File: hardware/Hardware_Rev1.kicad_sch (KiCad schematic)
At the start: 146 parts, among them J1 RJ45_LED_Shielded, J2 6P6C, Q1 BSS138, Q10 AO3401A, Q11 AO3401A, Q12 AO3401A, Q13 BSS138, Q14 BSS138, Q15 BSS138, Q16 AO3401A, Q17 AO3401A, Q18 AO3401A, Q19 BSS138, Q2 BSS138, Q20 BSS138, Q21 BSS138, Q22 AO3401A, Q23 AO3401A, Q24 AO3401A, Q3 BSS138, Q4 AO3401A, Q5 AO3401A, Q6 AO3401A, Q7 BSS138, Q8 BSS138, Q9 BSS138, U1 OKI, U2 Teensy4.1_DEV-16771

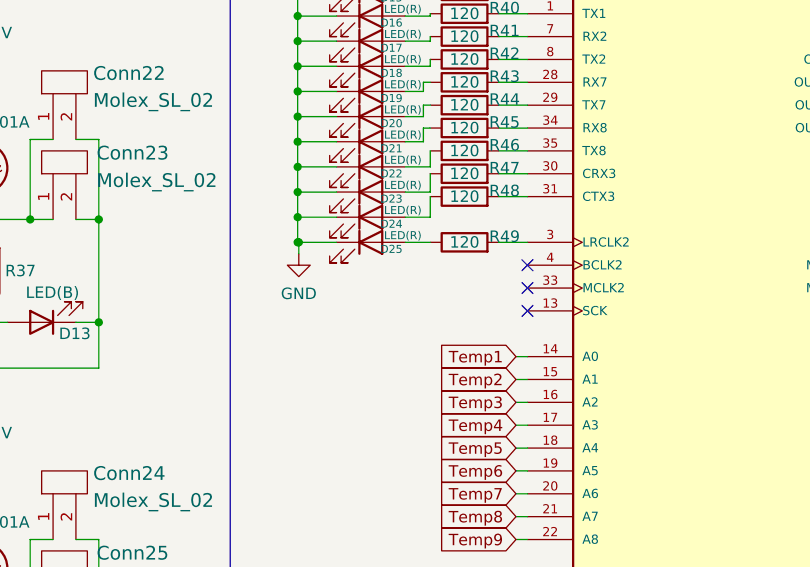
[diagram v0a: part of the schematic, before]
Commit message: Finished connections
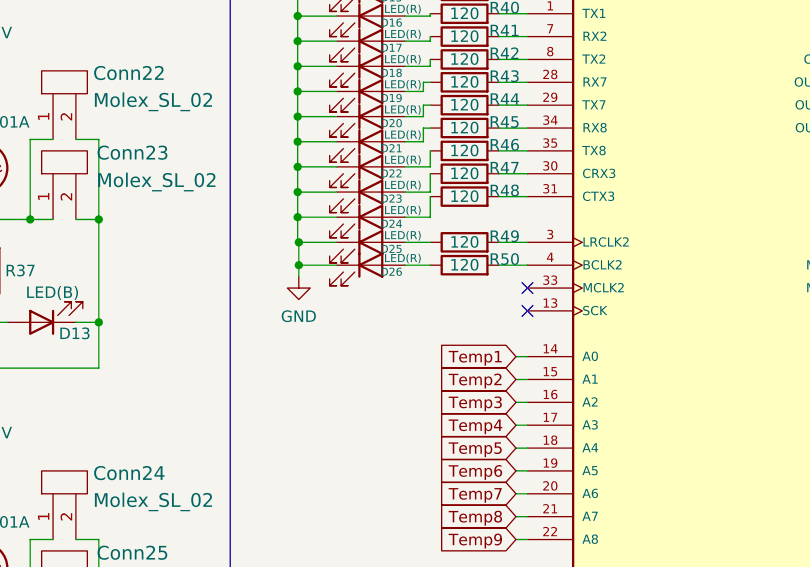
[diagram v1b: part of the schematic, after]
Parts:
- added D26: LED(R), LED_SMD:LED_0603_1608Metric_Pad1.05x0.95mm_HandSolder, symbol Device:LED
- added R50: 120, Resistor_SMD:R_0603_1608Metric_Pad0.98x0.95mm_HandSolder, symbol Device:R
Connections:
- net GND: now also D26.1 (K)
- net at U2.4 (BCLK2): now also R50.2
- new net: D26.2 (A), R50.1
- no-connect marks 23 -> 22
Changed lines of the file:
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@@
   (junction (at 187.833 77.216) (diameter 0) (color 0 0 0 0)
   )
+  (junction (at 187.96 82.55) (diameter 0) (color 0 0 0 0)
+  )
   (junction (at 73.66 63.5) (diameter 0) (color 0 0 0 0)
   )
@@
   (junction (at 102.235 93.98) (diameter 0) (color 0 0 0 0)
   )
-  (junction (at 187.96 80.01) (diameter 0) (color 0 0 0 0)
-  )
   (junction (at 125.095 167.005) (diameter 0) (color 0 0 0 0)
   )
@@
   (junction (at 33.655 63.5) (diameter 0) (color 0 0 0 0)
   )
-  (junction (at 187.833 80.01) (diameter 0) (color 0 0 0 0)
-  )
   (junction (at 153.035 153.035) (diameter 0) (color 0 0 0 0)
   )
@@
   (junction (at 45.72 121.92) (diameter 0) (color 0 0 0 0)
   )
+  (junction (at 187.96 80.01) (diameter 0) (color 0 0 0 0)
+  )
   (junction (at 22.225 116.205) (diameter 0) (color 0 0 0 0)
   )
@@
   (no_connect (at 254 31.75))
   (no_connect (at 254 29.21))
-  (no_connect (at 213.36 82.55))
   (no_connect (at 254 77.47))
   (no_connect (at 254 74.93))
@@
     (stroke (width 0) (type default) (color 0 0 0 0))
   )
+  (wire (pts (xy 187.96 80.01) (xy 187.96 82.55))
+    (stroke (width 0) (type default) (color 0 0 0 0))
+  )
   (wire (pts (xy 118.11 68.58) (xy 120.65 68.58))
     (stroke (width 0) (type default) (color 0 0 0 0))
@@
     (stroke (width 0) (type default) (color 0 0 0 0))
   )
+  (wire (pts (xy 192.151 82.55) (xy 187.96 82.55))
+    (stroke (width 0) (type default) (color 0 0 0 0))
+  )
   (wire (pts (xy 153.67 60.325) (xy 153.67 63.5))
     (stroke (width 0) (type default) (color 0 0 0 0))
@@
     (stroke (width 0) (type default) (color 0 0 0 0))
   )
+  (wire (pts (xy 199.771 82.55) (xy 202.565 82.55))
+    (stroke (width 0) (type default) (color 0 0 0 0))
+  )
   (wire (pts (xy 85.725 77.47) (xy 85.725 68.58))
     (stroke (width 0) (type default) (color 0 0 0 0))
@@
     (stroke (width 0) (type default) (color 0 0 0 0))
   )
-  (wire (pts (xy 187.96 80.01) (xy 187.833 80.01))
-    (stroke (width 0) (type default) (color 0 0 0 0))
-  )
   (wire (pts (xy 153.035 178.435) (xy 154.94 178.435))
     (stroke (width 0) (type default) (color 0 0 0 0))
@@
     (stroke (width 0) (type default) (color 0 0 0 0))
   )
+  (wire (pts (xy 210.185 82.55) (xy 213.36 82.55))
+    (stroke (width 0) (type default) (color 0 0 0 0))
+  )
   (wire (pts (xy 42.545 167.005) (xy 45.085 167.005))
     (stroke (width 0) (type default) (color 0 0 0 0))
@@
     (stroke (width 0) (type default) (color 0 0 0 0))
   )
-  (wire (pts (xy 187.96 80.01) (xy 187.96 81.28))
+  (wire (pts (xy 187.96 82.55) (xy 187.96 83.82))
     (stroke (width 0) (type default) (color 0 0 0 0))
   )
@@
     (stroke (width 0) (type default) (color 0 0 0 0))
   )
-  (wire (pts (xy 192.151 80.01) (xy 187.96 80.01))
+  (wire (pts (xy 187.833 80.01) (xy 187.96 80.01))
     (stroke (width 0) (type default) (color 0 0 0 0))
   )
@@
     (stroke (width 0) (type default) (color 0 0 0 0))
   )
+  (wire (pts (xy 187.96 80.01) (xy 192.151 80.01))
+    (stroke (width 0) (type default) (color 0 0 0 0))
+  )
   (wire (pts (xy 33.655 131.445) (xy 33.655 133.35))
     (stroke (width 0) (type default) (color 0 0 0 0))
@@
     (pin "1")
   )
+  (symbol (lib_id "Device:LED") (at 195.961 82.55 0) (unit 1)
+    (in_bom yes) (on_board yes)
+    (property "Reference" "D26" (id 0) (at 198.247 83.312 0)
+      (effects (font (size 0.889 0.889)))
+    )
+    (property "Value" "LED(R)" (id 1) (at 199.517 81.788 0)
+      (effects (font (size 0.889 0.889)))
+    )
+    (property "Footprint" "LED_SMD:LED_0603_1608Metric_Pad1.05x0.95mm_HandSolder" (id 2) (at 195.961 82.55 0)
+      (effects (font (size 1.27 1.27)) hide)
+    )
+    (property "Datasheet" "~" (id 3) (at 195.961 82.55 0)
+      (effects (font (size 1.27 1.27)) hide)
+    )
+    (pin "1")
+    (pin "2")
+  )
   (symbol (lib_id "power:GND") (at 337.82 89.535 0) (unit 1)
     (in_bom yes) (on_board yes) (fields_autoplaced)
@@
     (pin "1")
   )
-  (symbol (lib_id "power:GND") (at 187.96 81.28 0) (unit 1)
+  (symbol (lib_id "power:GND") (at 187.96 83.82 0) (unit 1)
     (in_bom yes) (on_board yes) (fields_autoplaced)
-    (property "Reference" "#PWR031" (id 0) (at 187.96 87.63 0)
+    (property "Reference" "#PWR031" (id 0) (at 187.96 90.17 0)
       (effects (font (size 1.27 1.27)) hide)
     )
-    (property "Value" "GND" (id 1) (at 187.96 85.7234 0))
-    (property "Footprint" "" (id 2) (at 187.96 81.28 0)
+    (property "Value" "GND" (id 1) (at 187.96 88.2634 0))
+    (property "Footprint" "" (id 2) (at 187.96 83.82 0)
       (effects (font (size 1.27 1.27)) hide)
     )
-    (property "Datasheet" "" (id 3) (at 187.96 81.28 0)
+    (property "Datasheet" "" (id 3) (at 187.96 83.82 0)
       (effects (font (size 1.27 1.27)) hide)
     )
@@
     (pin "2")
   )
+  (symbol (lib_id "Device:R") (at 206.375 82.55 90) (unit 1)
+    (in_bom yes) (on_board yes)
+    (property "Reference" "R50" (id 0) (at 210.82 81.915 90))
+    (property "Value" "120" (id 1) (at 206.375 82.55 90))
+    (property "Footprint" "Resistor_SMD:R_0603_1608Metric_Pad0.98x0.95mm_HandSolder" (id 2) (at 206.375 84.328 90)
+      (effects (font (size 1.27 1.27)) hide)
+    )
+    (property "Datasheet" "~" (id 3) (at 206.375 82.55 0)
+      (effects (font (size 1.27 1.27)) hide)
+    )
+    (pin "1")
+    (pin "2")
+  )
   (symbol (lib_id "Device:LED") (at 39.37 88.9 180) (unit 1)
     (in_bom yes) (on_board yes)
@@
       (reference "D25") (unit 1) (value "LED(R)") (footprint "LED_SMD:LED_0603_1608Metric_Pad1.05x0.95mm_HandSolder")
     )
+    (path "/6d949603-847f-4e56-b193-01912840b2f5"
+      (reference "D26") (unit 1) (value "LED(R)") (footprint "LED_SMD:LED_0603_1608Metric_Pad1.05x0.95mm_HandSolder")
+    )
     (path "/c2380cb7-4961-4052-bc8b-0b990bf9ca9f"
       (reference "J1") (unit 1) (value "RJ45_LED_Shielded") (footprint "MRDT_Connectors:RJ45_Teensy")
@@
       (reference "R49") (unit 1) (value "120") (footprint "Resistor_SMD:R_0603_1608Metric_Pad0.98x0.95mm_HandSolder")
     )
+    (path "/a6972e9c-2b36-4d0d-8530-9b703b7ced0d"
+      (reference "R50") (unit 1) (value "120") (footprint "Resistor_SMD:R_0603_1608Metric_Pad0.98x0.95mm_HandSolder")
+    )
     (path "/1a6178a5-56d4-4943-9131-ec94d86ded73"
